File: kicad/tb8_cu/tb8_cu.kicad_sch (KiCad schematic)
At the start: 10 parts, among them J1 Conn_02x25_Counter_Clockwise, U1 74AHCT74, U2 74AHCT08, U3 74AHCT32, U4 74AHCT573, U5 74AHCT238, U6 74AHCT238, U7 74AHCT573, U8 74AHCT00, U9 74AHCT573

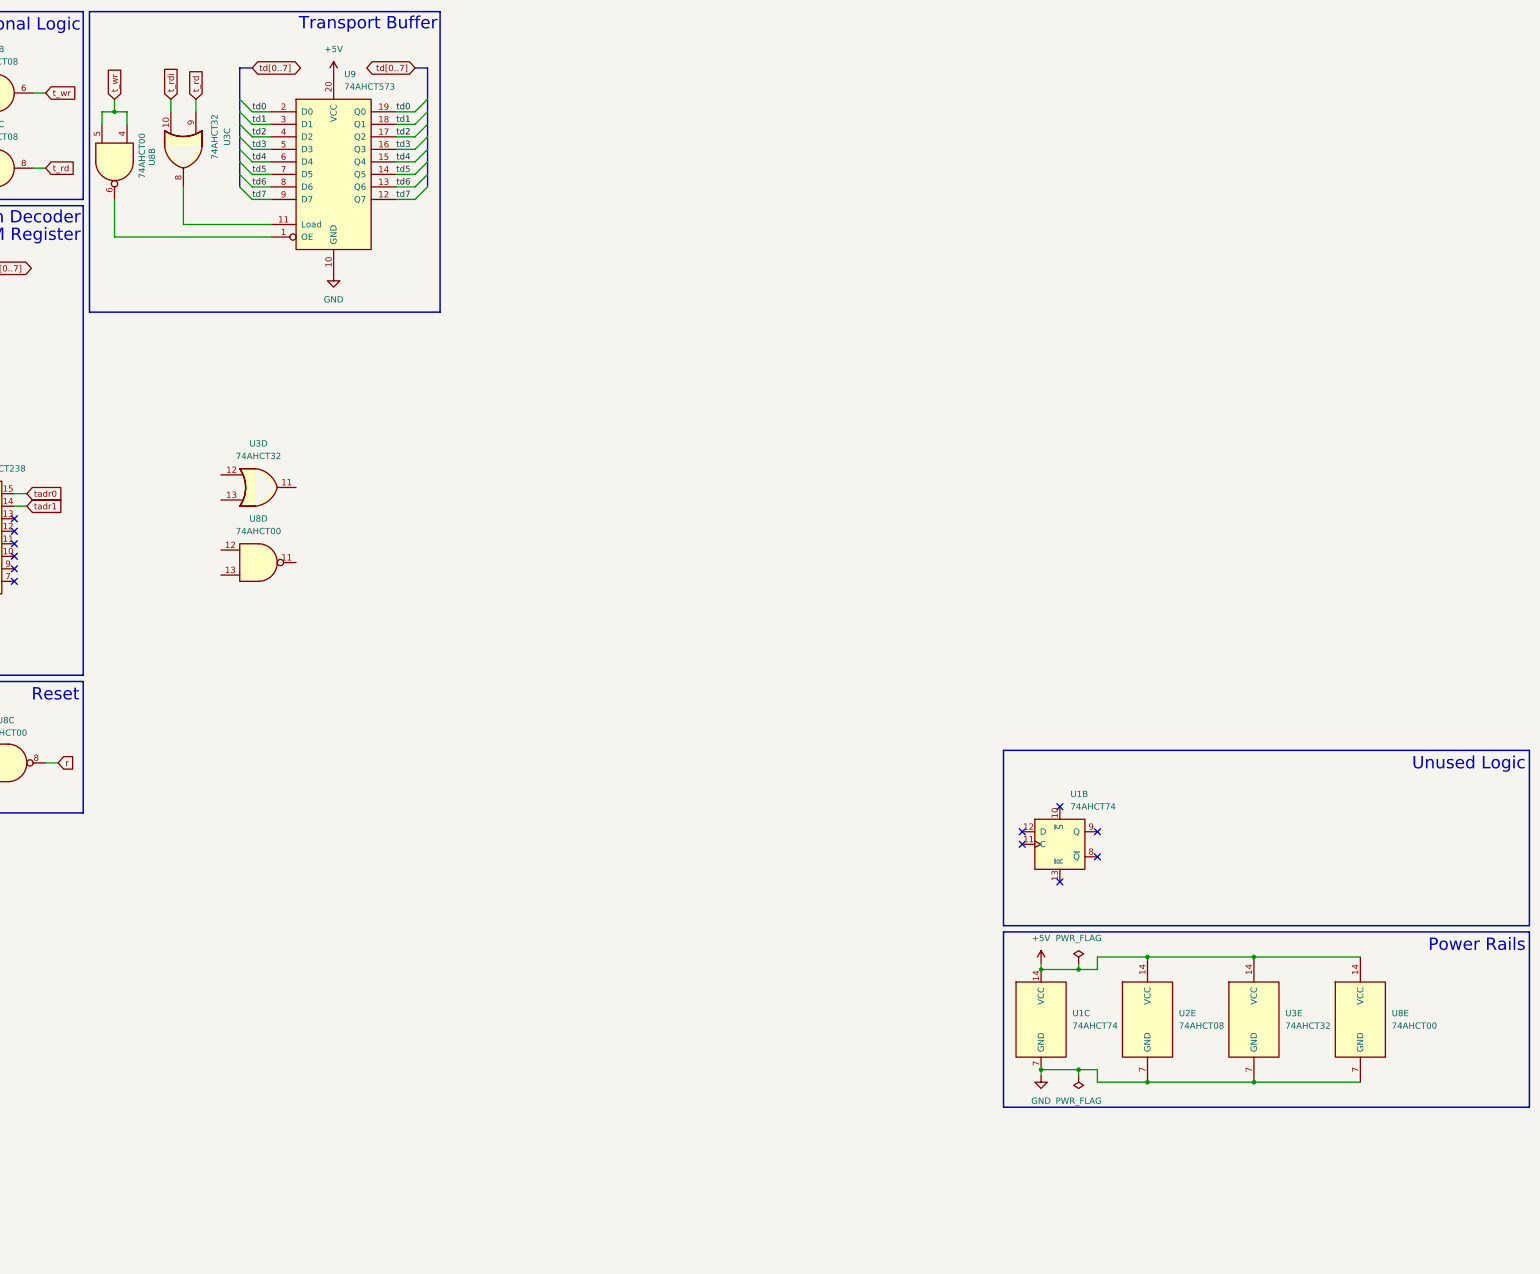
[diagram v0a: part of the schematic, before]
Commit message: tb8_cu sch&pcb in progress
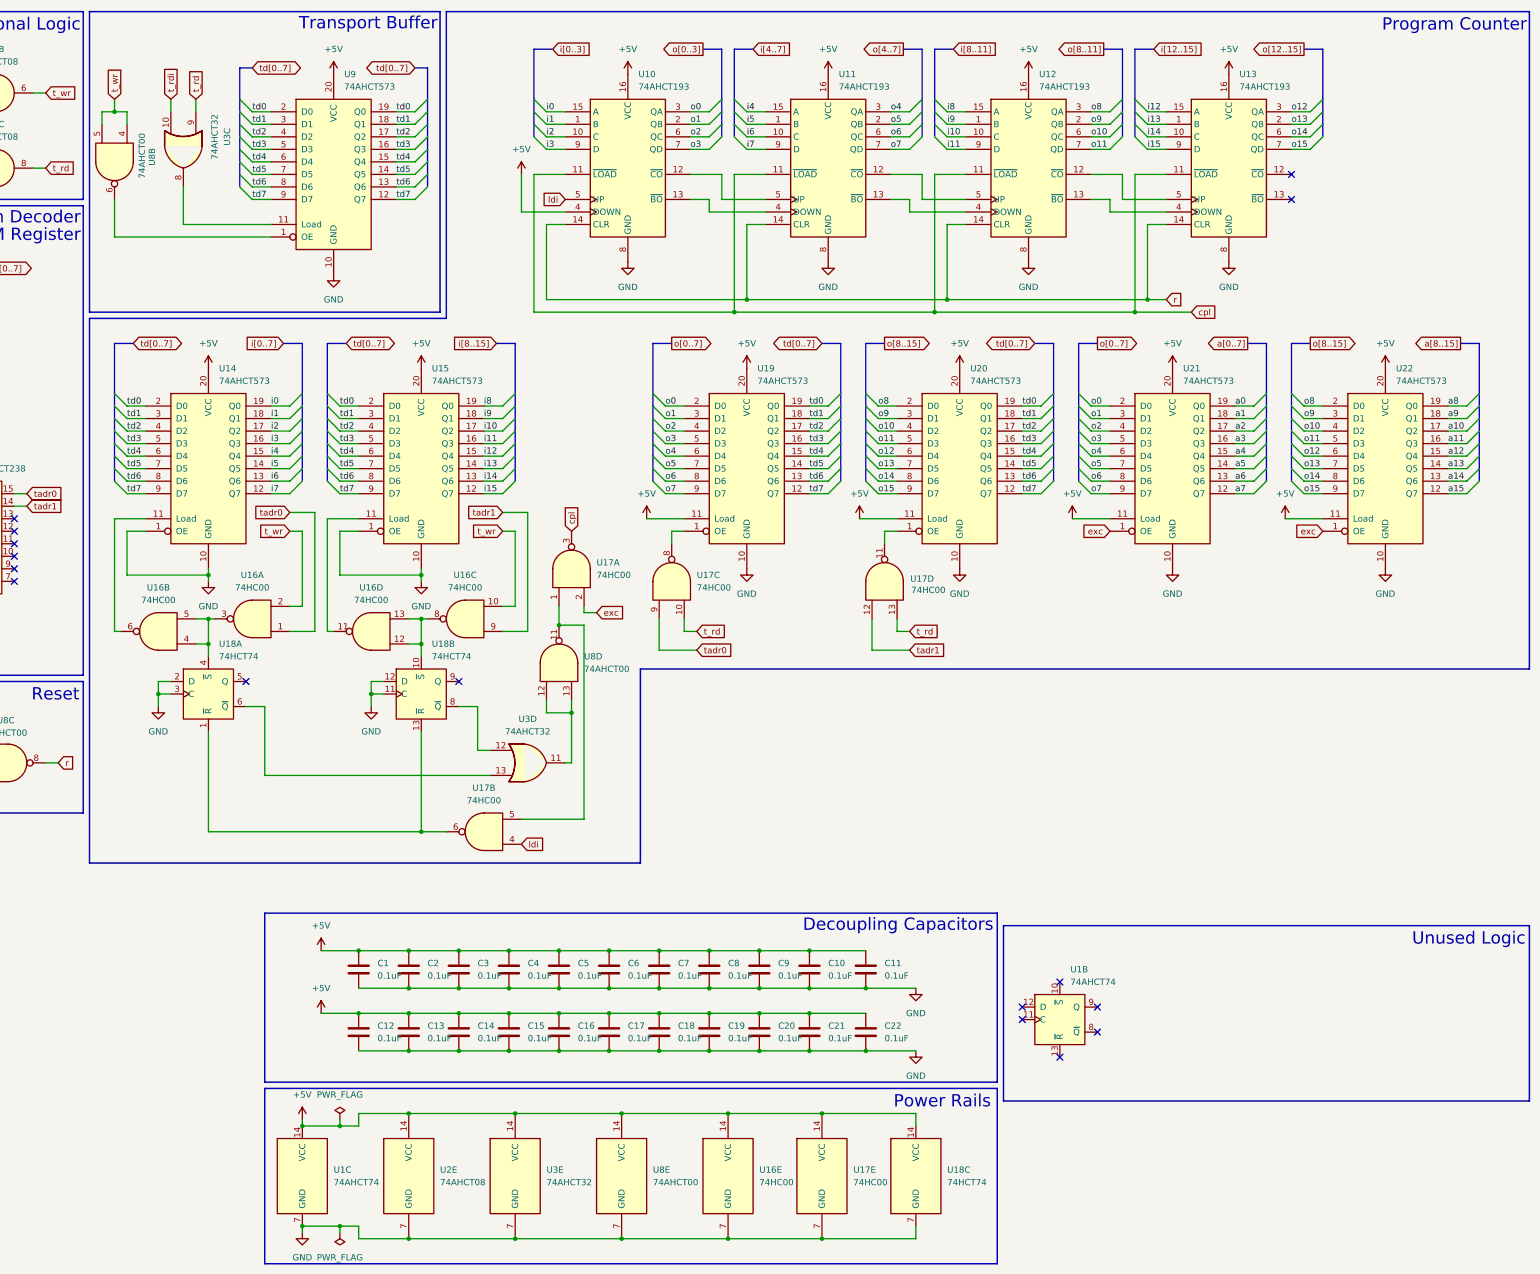
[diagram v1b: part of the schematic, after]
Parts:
- added C1, C10, C11, C12, C13, C14, C15, C16, C17, C18, C19, C2, C20, C21, C22, C3, C4, C5, C6, C7, C8, C9: 0.1uF, Capacitor_THT:C_Rect_L4.0mm_W2.5mm_P2.50mm, symbol Device:C
- added U10, U11, U12, U13: 74AHCT193, Package_DIP:DIP-16_W7.62mm_Socket_LongPads, symbol 74xx:74HCT193
- added U14, U15, U19, U20, U21, U22: 74AHCT573, Package_DIP:DIP-20_W7.62mm_Socket_LongPads, symbol 74xx:74LS573
- added U16, U17: 74HC00, Package_DIP:DIP-14_W7.62mm_Socket_LongPads, symbol 74xx:74HC00
- added U18: 74HCT74, Package_DIP:DIP-14_W7.62mm_Socket_LongPads, symbol 74xx:74HCT74
- J1: footprint (none) -> Custom_PCBEdge:25_2.54spacing
- U1, U2, U3, U8: footprint (none) -> Package_DIP:DIP-14_W7.62mm_Socket_LongPads
- U4, U7, U9: footprint (none) -> Package_DIP:DIP-20_W7.62mm_Socket_LongPads
- U5, U6: footprint (none) -> Package_DIP:DIP-16_W7.62mm_Socket_LongPads
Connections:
- net +5V: now also C1.1, C10.1, C11.1, C12.1, C13.1, C14.1, C15.1, C16.1, C17.1, C18.1, C19.1, C2.1, C20.1, C21.1, C22.1, C3.1, C4.1, C5.1, C6.1, C7.1, C8.1, C9.1, U10.16 (VCC), U10.4 (DOWN), U11.16 (VCC), U12.16 (VCC), U13.16 (VCC), U14.20 (VCC), U15.20 (VCC), U16.14 (VCC), U17.14 (VCC), U18.14 (VCC), U19.11 (Load), U19.20 (VCC), U20.11 (Load), U20.20 (VCC), U21.11 (Load), U21.20 (VCC), U22.11 (Load), U22.20 (VCC)
- net GND: now also C1.2, C10.2, C11.2, C12.2, C13.2, C14.2, C15.2, C16.2, C17.2, C18.2, C19.2, C2.2, C20.2, C21.2, C22.2, C3.2, C4.2, C5.2, C6.2, C7.2, C8.2, C9.2, U10.8 (GND), U11.8 (GND), U12.8 (GND), U13.8 (GND), U14.1 (OE), U14.10 (GND), U15.1 (OE), U15.10 (GND), U16.7 (GND), U17.7 (GND), U18.11 (C), U18.12 (D), U18.2 (D), U18.3 (C), U18.7 (GND), U19.10 (GND), U20.10 (GND), U21.10 (GND), U22.10 (GND)
- net a0: now also U21.19 (Q0)
- net a1: now also U21.18 (Q1)
- net a10: now also U22.17 (Q2)
- net a11: now also U22.16 (Q3)
- net a12: now also U22.15 (Q4)
- net a13: now also U22.14 (Q5)
- net a14: now also U22.13 (Q6)
- net a15: now also U22.12 (Q7)
- net a2: now also U21.17 (Q2)
- net a3: now also U21.16 (Q3)
- net a4: now also U21.15 (Q4)
- net a5: now also U21.14 (Q5)
- net a6: now also U21.13 (Q6)
- net a7: now also U21.12 (Q7)
- net a8: now also U22.19 (Q0)
- net a9: now also U22.18 (Q1)
- net exc: now also U17.2, U21.1 (OE), U22.1 (OE)
- net ldi: now also U10.5 (UP), U17.4
- net r: now also U10.14 (CLR), U11.14 (CLR), U12.14 (CLR), U13.14 (CLR)
- net t_rd: now also U17.10, U17.13
- net t_wr: now also U16.10, U16.2
- net tadr0: now also U16.1, U17.9
- net tadr1: now also U16.9, U17.12
- net td0: now also U14.2 (D0), U15.2 (D0), U19.19 (Q0), U20.19 (Q0)
- net td1: now also U14.3 (D1), U15.3 (D1), U19.18 (Q1), U20.18 (Q1)
- net td2: now also U14.4 (D2), U15.4 (D2), U19.17 (Q2), U20.17 (Q2)
- net td3: now also U14.5 (D3), U15.5 (D3), U19.16 (Q3), U20.16 (Q3)
- net td4: now also U14.6 (D4), U15.6 (D4), U19.15 (Q4), U20.15 (Q4)
- net td5: now also U14.7 (D5), U15.7 (D5), U19.14 (Q5), U20.14 (Q5)
- net td6: now also U14.8 (D6), U15.8 (D6), U19.13 (Q6), U20.13 (Q6)
- net td7: now also U14.9 (D7), U15.9 (D7), U19.12 (Q7), U20.12 (Q7)
- net at U3.11: now also U8.12, U8.13
- net at U3.12: now also U18.8 (~{Q})
- net at U3.13: now also U18.6 (~{Q})
- net at U8.11: now also U17.1, U17.5
- new net: U12.12 (~{CO}), U13.5 (UP)
- new net: U12.13 (~{BO}), U13.4 (DOWN)
- new net: U11.13 (~{BO}), U12.4 (DOWN)
- new net: U11.12 (~{CO}), U12.5 (UP)
- new net: U16.3, U16.4, U16.5, U18.4 (~{S})
- new net: U14.11 (Load), U16.6
- new net: U17.6, U18.1 (~{R}), U18.13 (~{R})
- new net: U17.11, U20.1 (OE)
- new net: U10.12 (~{CO}), U11.5 (UP)
- new net: U10.13 (~{BO}), U11.4 (DOWN)
- new net: U15.11 (Load), U16.11
- new net: U16.12, U16.13, U16.8, U18.10 (~{S})
- new net: U17.8, U19.1 (OE)
- new net cpl: U10.11 (~{LOAD}), U11.11 (~{LOAD}), U12.11 (~{LOAD}), U13.11 (~{LOAD}), U17.3
- new net i0: U10.15 (A), U14.19 (Q0)
- new net i1: U10.1 (B), U14.18 (Q1)
- new net i10: U12.10 (C), U15.17 (Q2)
- new net i11: U12.9 (D), U15.16 (Q3)
- new net i12: U13.15 (A), U15.15 (Q4)
- new net i13: U13.1 (B), U15.14 (Q5)
- new net i14: U13.10 (C), U15.13 (Q6)
- new net i15: U13.9 (D), U15.12 (Q7)
- new net i2: U10.10 (C), U14.17 (Q2)
- new net i3: U10.9 (D), U14.16 (Q3)
- new net i4: U11.15 (A), U14.15 (Q4)
- new net i5: U11.1 (B), U14.14 (Q5)
- new net i6: U11.10 (C), U14.13 (Q6)
- new net i7: U11.9 (D), U14.12 (Q7)
- new net i8: U12.15 (A), U15.19 (Q0)
- new net i9: U12.1 (B), U15.18 (Q1)
- new net o0: U10.3 (QA), U19.2 (D0), U21.2 (D0)
- new net o1: U10.2 (QB), U19.3 (D1), U21.3 (D1)
- new net o10: U12.6 (QC), U20.4 (D2), U22.4 (D2)
- new net o11: U12.7 (QD), U20.5 (D3), U22.5 (D3)
- new net o12: U13.3 (QA), U20.6 (D4), U22.6 (D4)
- new net o13: U13.2 (QB), U20.7 (D5), U22.7 (D5)
- new net o14: U13.6 (QC), U20.8 (D6), U22.8 (D6)
- new net o15: U13.7 (QD), U20.9 (D7), U22.9 (D7)
- new net o2: U10.6 (QC), U19.4 (D2), U21.4 (D2)
- new net o3: U10.7 (QD), U19.5 (D3), U21.5 (D3)
- new net o4: U11.3 (QA), U19.6 (D4), U21.6 (D4)
- new net o5: U11.2 (QB), U19.7 (D5), U21.7 (D5)
- new net o6: U11.6 (QC), U19.8 (D6), U21.8 (D6)
- new net o7: U11.7 (QD), U19.9 (D7), U21.9 (D7)
- new net o8: U12.3 (QA), U20.2 (D0), U22.2 (D0)
- new net o9: U12.2 (QB), U20.3 (D1), U22.3 (D1)
- no-connect marks 16 -> 20
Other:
- note added: "Decoupling Capacitors"
- note added: "Program Counter"
- title: (none) -> tb8 Control Unit Card
- moved on the sheet: U1B, U1C, U2E, U3D, U3E, U8D, U8E
